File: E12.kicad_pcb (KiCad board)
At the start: 4 copper layers, 16.3 x 6.2 mm, 20 parts, among them J3 59453-061110EDHLF, U1 WS2811, U2 WS2811, U3 WS2811, U4 WS2811

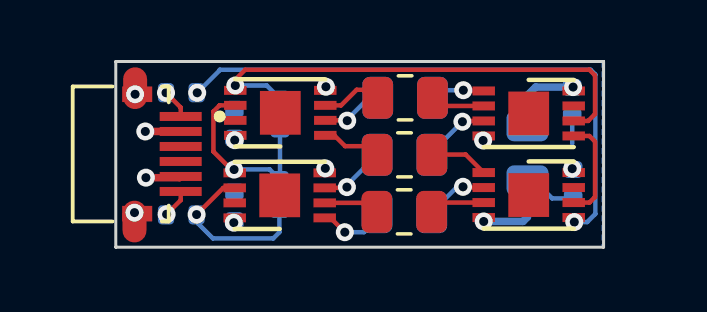
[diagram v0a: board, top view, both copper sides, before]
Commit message: Initial commit
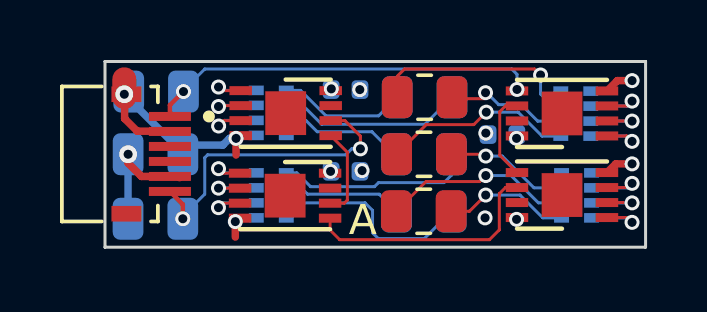
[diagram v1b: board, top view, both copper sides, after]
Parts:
- removed C4: 100n, Capacitor_SMD:C_0402_1005Metric
- removed R10: 0, Resistor_SMD:R_0402_1005Metric
- removed R7, R8: 160, Resistor_SMD:R_0402_1005Metric
- added R12: R, Resistor_SMD:R_0805_2012Metric, B.Cu at (135.9, 96.1)
- added RN1: R_Pack04, Resistor_SMD:R_Array_Concave_4x0402, B.Cu at (139.8, 92.5)
- added RN2: R_Pack04, Resistor_SMD:R_Array_Concave_4x0402, B.Cu at (139.8, 95.3)
- added RN3: R_Pack04, Resistor_SMD:R_Array_Concave_4x0402, B.Cu at (149.9, 92.6)
- added RN4: R_Pack04, Resistor_SMD:R_Array_Concave_4x0402, B.Cu at (150.0, 95.3)
- R11: value 0 -> R; footprint Resistor_SMD:R_0402_1005Metric -> Resistor_SMD:R_0805_2012Metric
- moved R9 12.4 mm to (135.9, 93.9), turned to 0 degrees
- moved C2 5.37 mm to (142.3, 91.8), turned to 0 degrees
- moved R11 4.20 mm to (136.0, 91.8), turned to 180 degrees
- moved C3 4.03 mm to (142.3, 94.5), turned to 0 degrees
- moved U3 2.94 mm to (149.5, 95.3), turned to 180 degrees
- moved U4 2.94 mm to (149.5, 92.6), turned to 180 degrees
- moved C1 2.87 mm to (147.5, 93.3), turned to 180 degrees
- moved U2 2.76 mm to (140.3, 95.3), turned to 0 degrees
- moved U1 2.75 mm to (140.3, 92.6), turned to 0 degrees
- moved R1 0.65 mm to (144.9, 92.0)
- moved R3 0.65 mm to (144.9, 95.8)
- moved R4 0.65 mm to (144.9, 92.0)
- moved R2 0.65 mm to (144.9, 93.9)
- moved R5 0.65 mm to (144.9, 93.9)
- moved R6 0.65 mm to (144.9, 95.8)
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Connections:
- J3 pad 1: Net-(J3-Pad1) -> DO
- J3 pad 6: Net-(J3-Pad6) -> DI
- R1 pad 1: OUT7 -> Port-10
- R1 pad 2: OUT5 -> Port-11
- R11 pad 1: Net-(R11-Pad1) -> DO
- R11 pad 2: Net-(R10-Pad1) -> GND
- R2 pad 1: OUT9 -> Port-8
- R2 pad 2: OUT3 -> Port-9
- R3 pad 1: OUT11 -> Port-6
- R3 pad 2: OUT1 -> Port-7
- R4 pad 1: OUT6 -> Port-1
- R4 pad 2: OUT4 -> Port-0
- R5 pad 1: OUT8 -> Port-3
- R5 pad 2: OUT2 -> Port-2
- R6 pad 1: OUT10 -> Port-5
- R6 pad 2: OUT0 -> Port-4
- U1 pad 5: Net-(R10-Pad1) -> Net-(U1-Pad5)
- U2 pad 5: Net-(R11-Pad1) -> Net-(U2-Pad5)
- U2 pad 6: Net-(R10-Pad1) -> Net-(U1-Pad5)
- U3 pad 6: Net-(R11-Pad1) -> Net-(U2-Pad5)
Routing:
- net Net-(R11-Pad1): track 16.3 -> 0.00 mm, vias 1 -> 0
- net Net-(U2-Pad5): track 0.00 -> 8.19 mm
- net Port-11: track 0.00 -> 7.14 mm, vias 0 -> 1
- net Port-5: track 0.00 -> 6.81 mm
- net Net-(R10-Pad1): track 6.56 -> 0.00 mm, vias 1 -> 0
- net Port-3: track 0.00 -> 6.55 mm
- net Port-9: track 0.00 -> 6.38 mm, vias 0 -> 1
- net Port-7: track 0.00 -> 6.38 mm, vias 0 -> 1
- net Port-1: track 0.00 -> 6.16 mm
- net DO: track 19.1 -> 13.1 mm
- net DI: track 5.64 -> 10.2 mm, vias 1 -> 2
- net Port-2: track 0.00 -> 4.54 mm
- net Port-0: track 0.00 -> 4.31 mm
- net Port-6: track 0.00 -> 4.22 mm, vias 0 -> 1
- net Port-10: track 0.00 -> 4.21 mm, vias 0 -> 1
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- added copper zone on F.Cu, net GND
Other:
- board size 16.3 x 6.2 mm -> 18 x 6.2 mm
- rule solder_mask_min_width: 0.08 -> 0.1
- board text added: "A"
- board text added: "B"
- board text removed: "0"
- board text removed: "10"
- board text removed: "2"
- board text removed: "4"
- board text removed: "6"
- board text removed: "8"
- board text removed: "E12"
- board text removed: "fs"
